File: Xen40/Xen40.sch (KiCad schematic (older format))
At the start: 23 parts

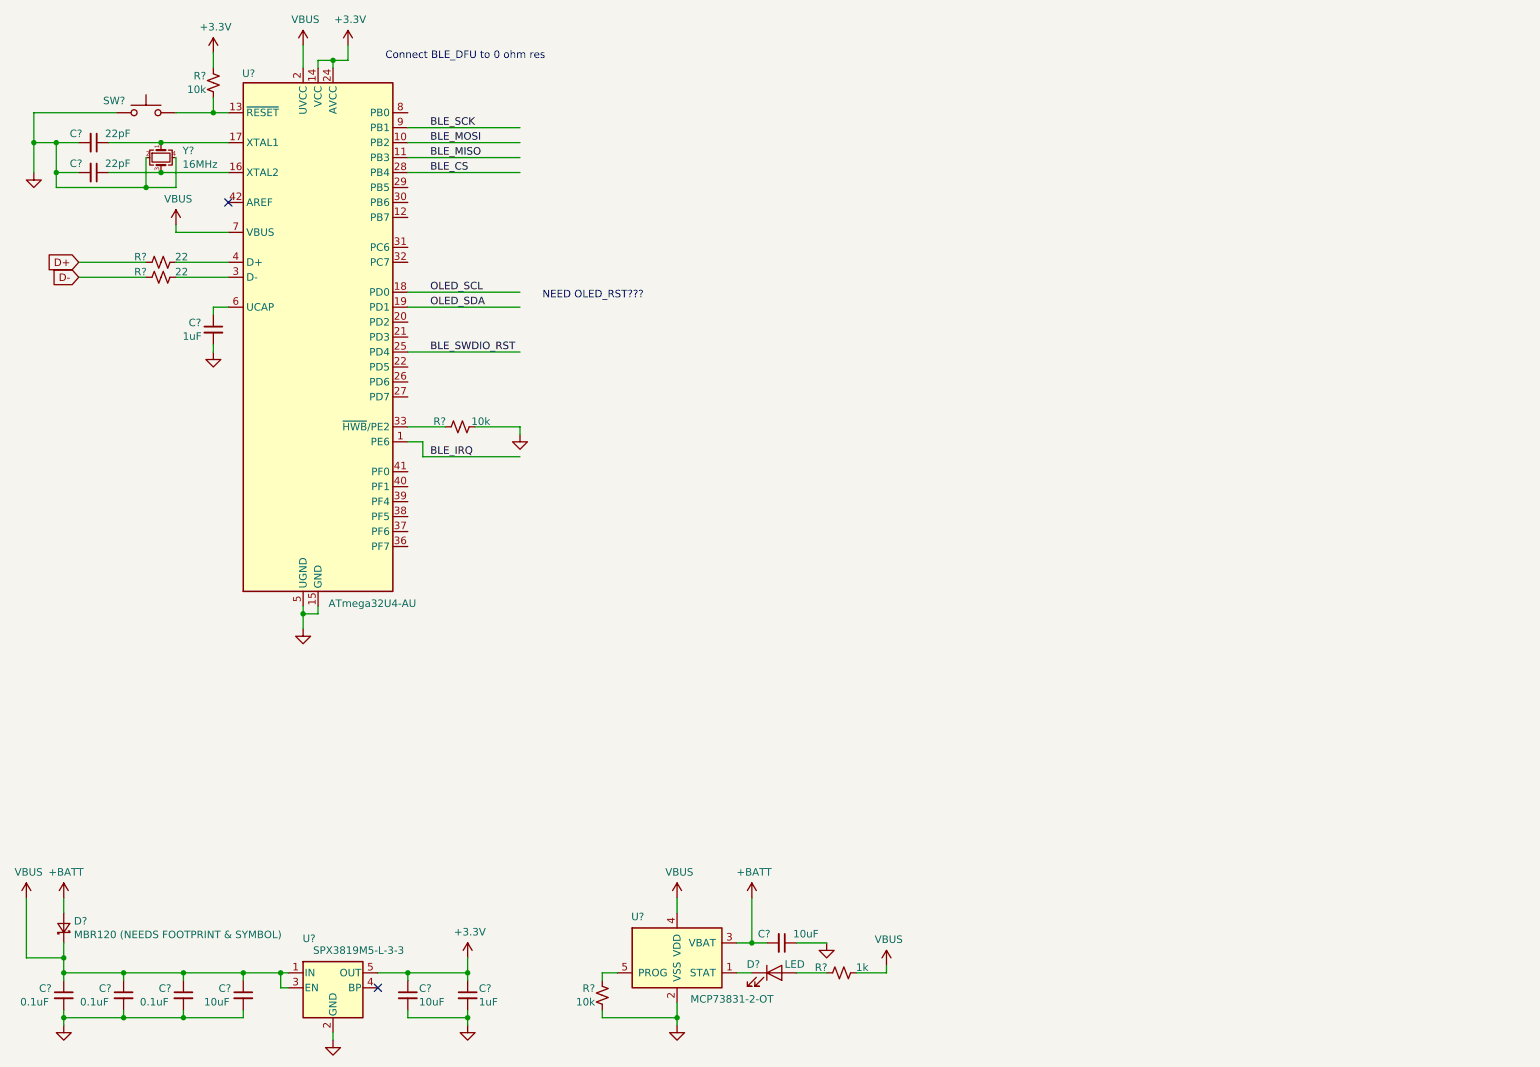
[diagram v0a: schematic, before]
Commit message: new files
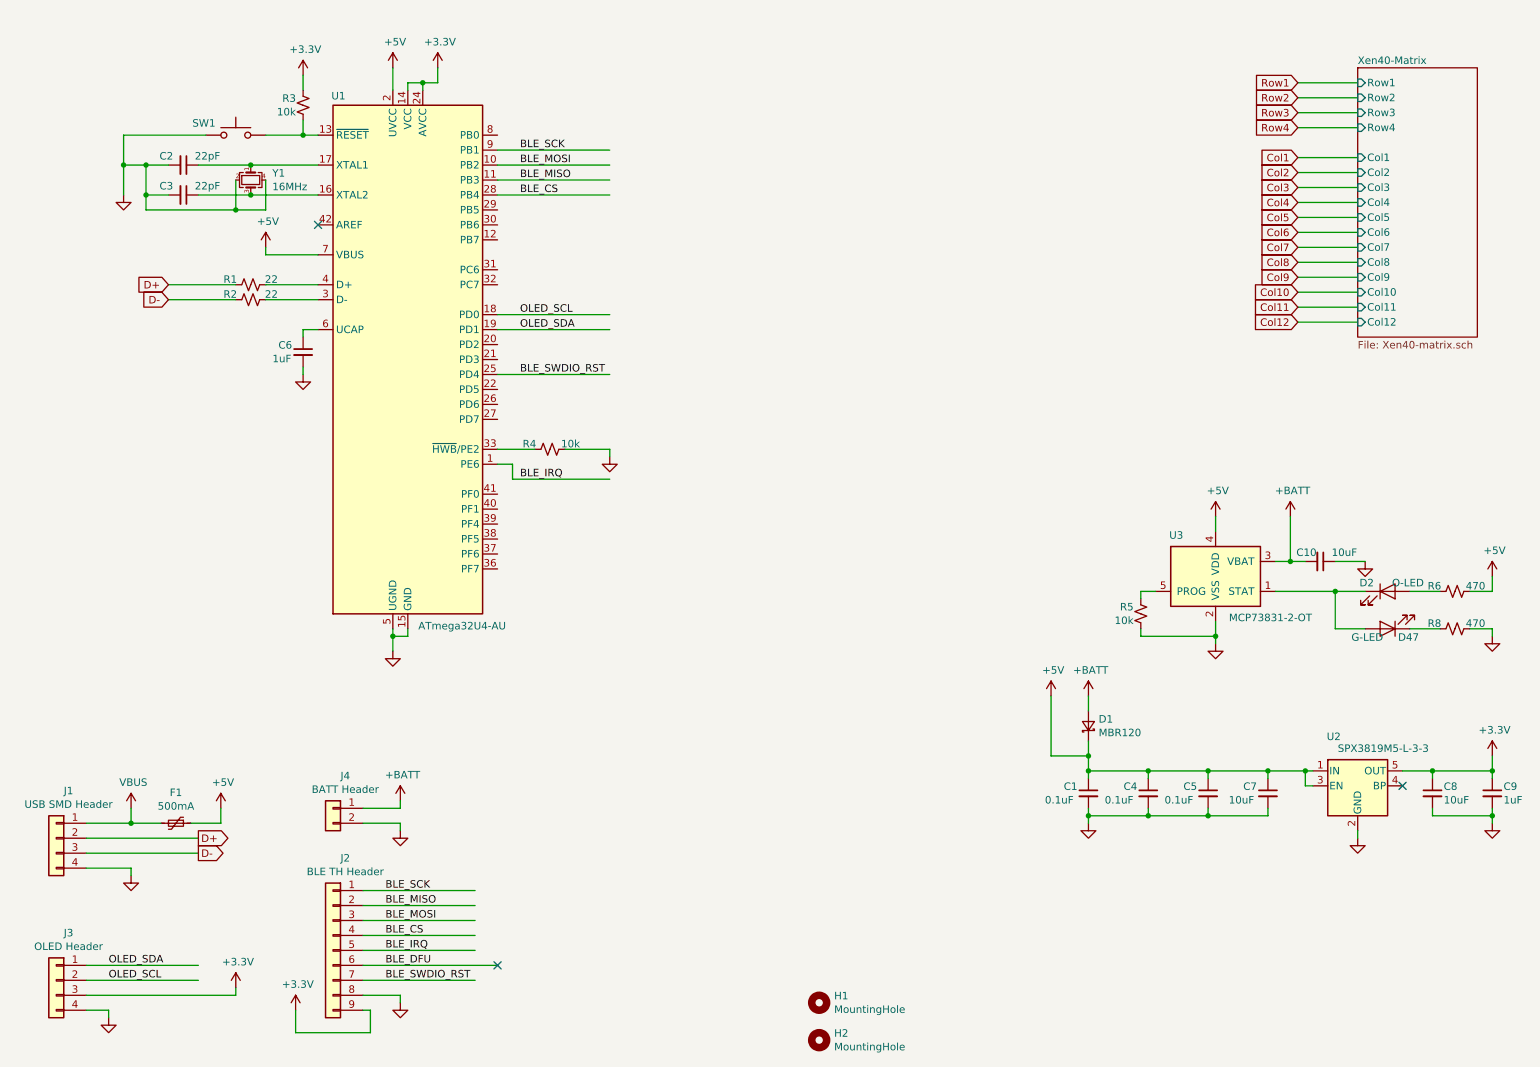
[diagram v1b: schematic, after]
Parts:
- added D47: G-LED, LED_SMD:LED_0805_2012Metric_Pad1.15x1.40mm_HandSolder, symbol Device:LED
- added F1: 500mA, Fuse:Fuse_1206_3216Metric_Pad1.42x1.75mm_HandSolder, symbol Device:Polyfuse_Small
- added H1, H2: MountingHole, random-keyboard-parts:MOUNTINGHOLE_2.5_PLATED, symbol Mechanical:MountingHole
- added J1: USB SMD Header, random-keyboard-parts:S4B-ZR, symbol Connector_Generic:Conn_01x04
- added J2: BLE TH Header, random-keyboard-parts:1X09_ROUND_70, symbol Connector_Generic:Conn_01x09
- added J3: OLED Header, random-keyboard-parts:OLED_4Pin, symbol Connector_Generic:Conn_01x04
- added J4: BATT Header, random-keyboard-parts:S2B-PH-K-S, symbol Connector_Generic:Conn_01x02
- added R8: 470, Resistor_SMD:R_0805_2012Metric_Pad1.15x1.40mm_HandSolder, symbol Device:R_Small_US
- C1, C10, C2, C3, C4, C5, C6, C7, C8, C9: renamed from C?; footprint (none) -> Capacitor_SMD:C_0805_2012Metric
- D1: renamed from D?; value MBR120 (NEEDS FOOTPRINT & SYMBOL) -> MBR120; footprint (none) -> Diode_SMD:D_SOD-123
- D2: renamed from D?; value LED -> O-LED; footprint (none) -> LED_SMD:LED_0805_2012Metric_Pad1.15x1.40mm_HandSolder
- R1, R2, R3, R4, R5: renamed from R?; footprint (none) -> Resistor_SMD:R_0805_2012Metric_Pad1.15x1.40mm_HandSolder
- R6: renamed from R?; value 1k -> 470; footprint (none) -> Resistor_SMD:R_0805_2012Metric_Pad1.15x1.40mm_HandSolder
- SW1: renamed from SW?; footprint (none) -> random-keyboard-parts:SKQG-1155865
- Y1: renamed from Y?; footprint (none) -> Crystal:Crystal_SMD_3225-4Pin_3.2x2.5mm_HandSoldering
- gave numbers to parts that had none: 3
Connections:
- net labels added: +5V, BLE_DFU, Col1, Col10, Col11, Col12, Col2, Col3, Col4, Col5, Col6, Col7, Col8, Col9, Row1, Row2, Row3, Row4
- wire segments 101 -> 155
- no-connect marks 2 -> 3
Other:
- note removed: "Connect BLE_DFU to 0 ohm res\n"
- note removed: "NEED OLED_RST???\n"
- moved on the sheet: C1, C10, C2, C3, C4, C5, C6, C7, C8, C9, D1, D2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
